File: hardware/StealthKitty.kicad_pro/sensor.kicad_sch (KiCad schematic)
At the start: 13 parts, among them J301 Conn_01x06, J302 Conn_01x06, J303 Conn_01x08, U301 ADXL343

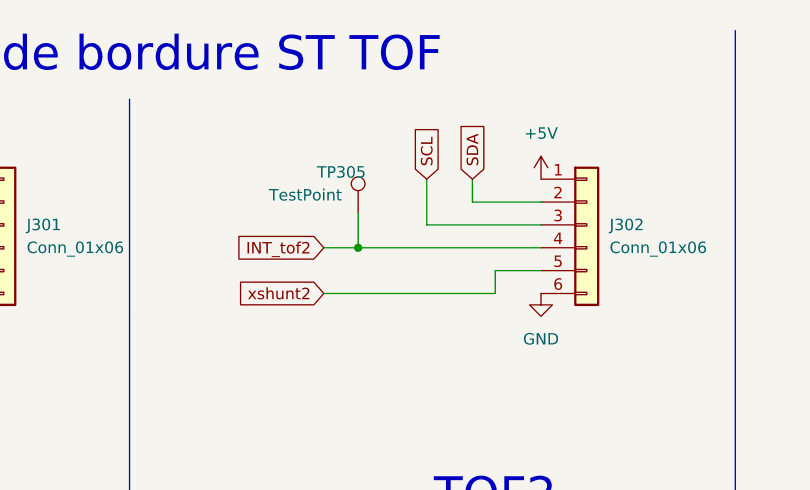
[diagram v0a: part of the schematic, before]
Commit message: Modification Placement 09/10/24
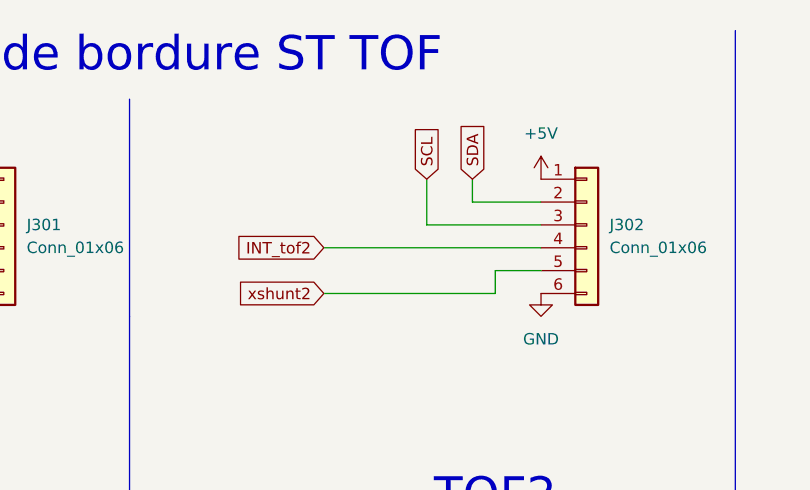
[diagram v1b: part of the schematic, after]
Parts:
- removed TP305: TestPoint, TestPoint:TestPoint_Pad_D1.5mm, symbol Connector:TestPoint
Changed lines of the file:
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@@
-	)
-	(junction
-		(at 102.87 36.83)
-		(diameter 0)
-		(color 0 0 0 0)
 	)
 	(junction
@@
 	(wire
 		(pts
-			(xy 102.87 36.83) (xy 123.19 36.83)
+			(xy 99.06 36.83) (xy 123.19 36.83)
 		)
 		(stroke
@@
 	(wire
 		(pts
-			(xy 99.06 36.83) (xy 102.87 36.83)
-		)
-		(stroke
-			(width 0)
-			(type default)
-		)
-	)
-	(wire
-		(pts
 			(xy 110.49 29.21) (xy 110.49 34.29)
 		)
@@
 		(pts
 			(xy 52.07 39.37) (xy 58.42 39.37)
-		)
-		(stroke
-			(width 0)
-			(type default)
-		)
-	)
-	(wire
-		(pts
-			(xy 102.87 33.02) (xy 102.87 36.83)
 		)
 		(stroke
@@
 					(unit 1)
 				)
-			)
-		)
-	)
-	(symbol
-		(lib_id "Connector:TestPoint")
-		(at 102.87 33.02 0)
-		(unit 1)
-		(exclude_from_sim no)
-		(in_bom yes)
-		(on_board yes)
-		(dnp no)
-		(property "Reference" "TP305"
-			(at 98.298 28.448 0)
-			(effects
-				(font
-					(size 1.27 1.27)
-				)
-				(justify left)
-			)
-		)
-		(property "Value" "TestPoint"
-			(at 92.964 30.988 0)
-			(effects
-				(font
-					(size 1.27 1.27)
-				)
-				(justify left)
-			)
-		)
-		(property "Footprint" "TestPoint:TestPoint_Pad_D1.5mm"
-			(at 107.95 33.02 0)
-			(effects
-				(font
-					(size 1.27 1.27)
-				)
-				(hide yes)
-			)
-		)
-		(property "Datasheet" "~"
-			(at 107.95 33.02 0)
-			(effects
-				(font
-					(size 1.27 1.27)
-				)
-				(hide yes)
-			)
-		)
-		(property "Description" "test point"
-			(at 102.87 33.02 0)
-			(effects
-				(font
-					(size 1.27 1.27)
-				)
-				(hide yes)
-			)
-		)
-		(pin "1"
-		)
-		(instances
-			(project "StealthKitty.kicad_pro"
-				(path "/23d5732b-7ccb-40aa-85a2-3b18421ac23b/8cd8413a-9ba4-4bd6-b413-2331caa50cc2"
-					(reference "TP305")
-					(unit 1)
-				)

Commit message: CRCR
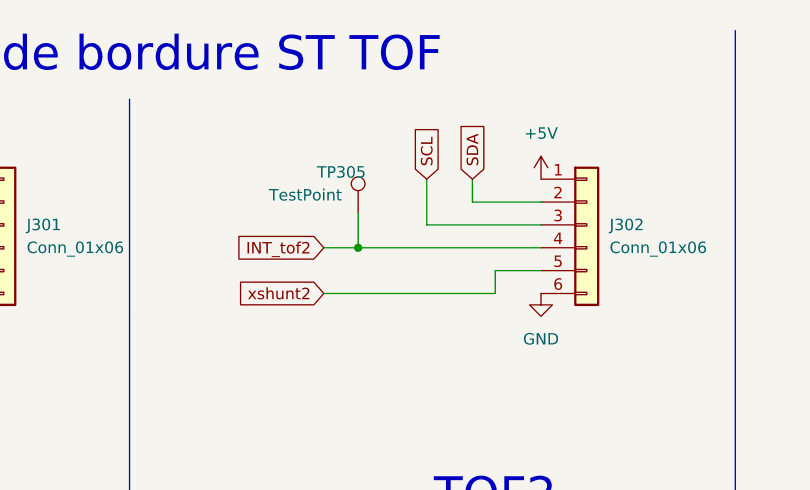
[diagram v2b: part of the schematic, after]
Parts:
- added TP305: TestPoint, TestPoint:TestPoint_Pad_D1.5mm, symbol Connector:TestPoint
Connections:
- net INT_tof2: now also TP305.1
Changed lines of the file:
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@@
+	)
+	(junction
+		(at 102.87 36.83)
+		(diameter 0)
+		(color 0 0 0 0)
 	)
 	(junction
@@
 	(wire
 		(pts
-			(xy 99.06 36.83) (xy 123.19 36.83)
+			(xy 102.87 36.83) (xy 123.19 36.83)
 		)
 		(stroke
@@
 	(wire
 		(pts
+			(xy 99.06 36.83) (xy 102.87 36.83)
+		)
+		(stroke
+			(width 0)
+			(type default)
+		)
+	)
+	(wire
+		(pts
 			(xy 110.49 29.21) (xy 110.49 34.29)
 		)
@@
 		(pts
 			(xy 52.07 39.37) (xy 58.42 39.37)
+		)
+		(stroke
+			(width 0)
+			(type default)
+		)
+	)
+	(wire
+		(pts
+			(xy 102.87 33.02) (xy 102.87 36.83)
 		)
 		(stroke
@@
 					(unit 1)
 				)
+			)
+		)
+	)
+	(symbol
+		(lib_id "Connector:TestPoint")
+		(at 102.87 33.02 0)
+		(unit 1)
+		(exclude_from_sim no)
+		(in_bom yes)
+		(on_board yes)
+		(dnp no)
+		(property "Reference" "TP305"
+			(at 98.298 28.448 0)
+			(effects
+				(font
+					(size 1.27 1.27)
+				)
+				(justify left)
+			)
+		)
+		(property "Value" "TestPoint"
+			(at 92.964 30.988 0)
+			(effects
+				(font
+					(size 1.27 1.27)
+				)
+				(justify left)
+			)
+		)
+		(property "Footprint" "TestPoint:TestPoint_Pad_D1.5mm"
+			(at 107.95 33.02 0)
+			(effects
+				(font
+					(size 1.27 1.27)
+				)
+				(hide yes)
+			)
+		)
+		(property "Datasheet" "~"
+			(at 107.95 33.02 0)
+			(effects
+				(font
+					(size 1.27 1.27)
+				)
+				(hide yes)
+			)
+		)
+		(property "Description" "test point"
+			(at 102.87 33.02 0)
+			(effects
+				(font
+					(size 1.27 1.27)
+				)
+				(hide yes)
+			)
+		)
+		(pin "1"
+		)
+		(instances
+			(project "StealthKitty.kicad_pro"
+				(path "/23d5732b-7ccb-40aa-85a2-3b18421ac23b/8cd8413a-9ba4-4bd6-b413-2331caa50cc2"
+					(reference "TP305")
+					(unit 1)
+				)
